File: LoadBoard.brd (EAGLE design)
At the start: 100 x 100 mm, 76 parts, among them IC1 7805TV, IC2 LM358D, IC3 MCP23S17SO, Q1 IRFZ44N, Q2 16MHz, T1 BC817, U1 ATMEGA328P_TQFP, U2 MAX232SOIC16

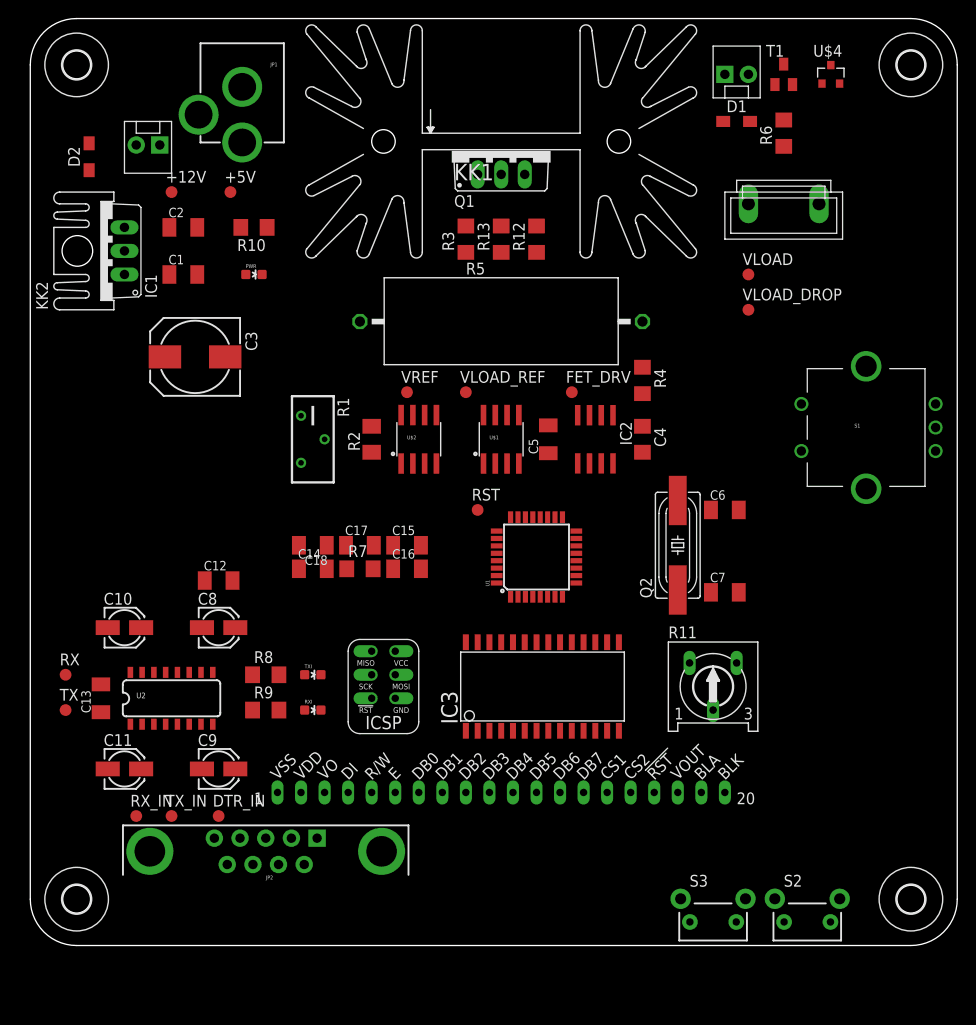
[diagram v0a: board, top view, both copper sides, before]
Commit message: routed first version of the board
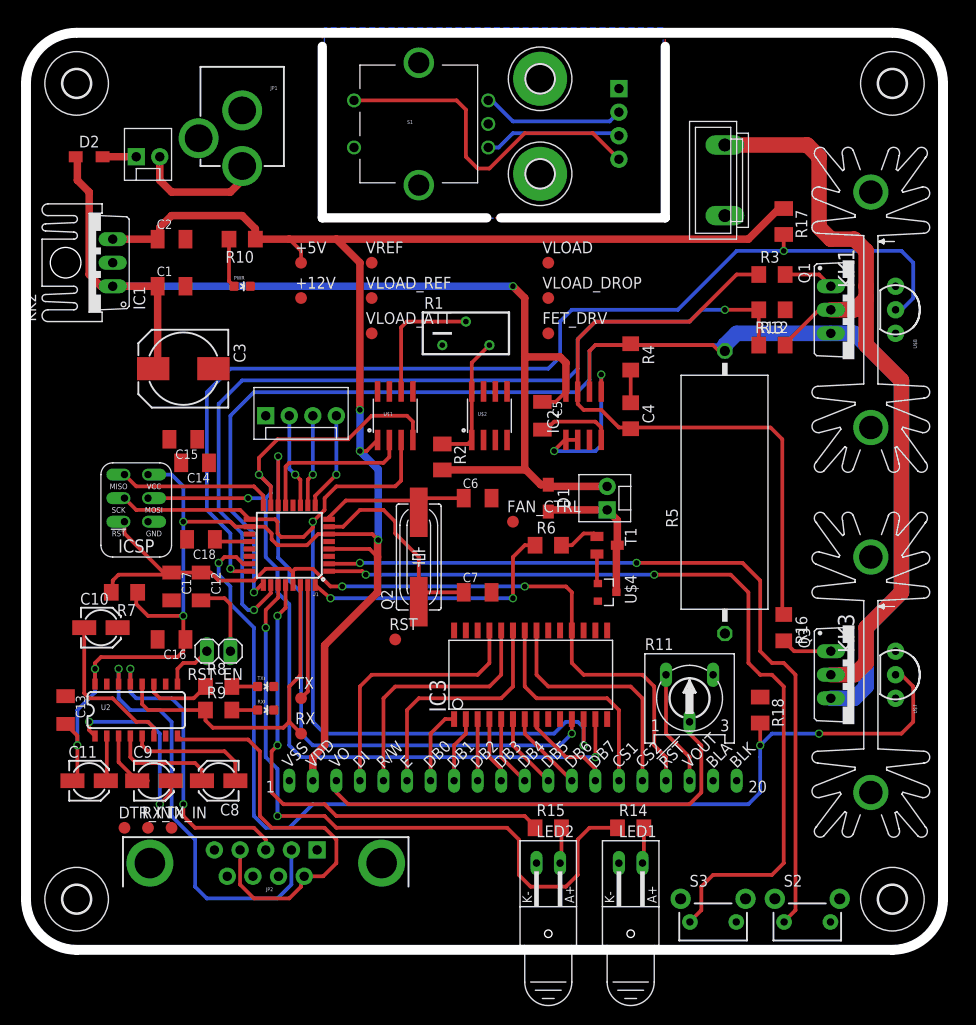
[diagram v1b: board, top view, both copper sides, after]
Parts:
- added ENCODER, JP3: (no value), SparkFun-Connectors:MOLEX-1X4
- added FAN_CTRL, VLOAD_ATT: TPB1,27, testpad:B1,27
- added H5, H6: 3MM, holes:3,0-PAD
- added KK3: SK104-PAD, heatsink:SK104-PAD
- added LED1, LED2: (no value), led:Q62902-B155
- added Q3: IRFZ44N, OwnStuff:TO-220-V
- added R14, R15, R16: 100, rcl:R1206
- added R17, R18: 4k7, rcl:M1206
- added RST_EN: (no value), pinhead:1X02
- added U$7, U$8: DS18B20, OwnStuff:TO-92
- KK1: value SK129 -> SK104-PAD; device heatsink:SK129-HOLE -> heatsink:SK104-PAD
- moved U$4 60.9 mm to (62.2, 38.1), turned to 270 degrees
- moved S1 58.3 mm to (41.9, 88.6)
- moved T1 54.3 mm to (62.2, 43.2), turned to 270 degrees
- moved R6 51.2 mm to (55.9, 43.2), turned to 0 degrees
- moved FAN 48.7 mm to (62.2, 47.0), turned to 90 degrees
- moved D1 45.4 mm to (55.9, 48.3), turned to 270 degrees
- moved KK1 44.9 mm to (91.4, 68.6), turned to 270 degrees
- moved Q1 38.4 mm to (86.4, 68.6), turned to 270 degrees
- moved R3 33.2 mm to (80.0, 72.4), turned to 0 degrees
- moved U$5 32.8 mm to (11.4, 48.3)
- moved R5 30.4 mm to (74.9, 48.9), turned to 90 degrees
- moved R13 30.2 mm to (80.0, 68.6), turned to 180 degrees
- moved Q2 28.0 mm to (41.9, 41.9)
- moved R12 27.9 mm to (80.0, 64.8), turned to 0 degrees
- moved C6 26.7 mm to (48.3, 48.3)
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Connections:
- new net GNDIO: JP3.1, S1.C, S1.SW-
- new net LED1: R14.1, U1.27
- new net LED2: R15.1, U1.28
- new net N$43: LED1.A, R14.2
- new net N$44: LED2.A, R15.2
- new net N$45: JP3.4, S1.SW+
- new net N$46: JP3.3, S1.A
- new net N$47: Q3.1, R16.2
- new net N$49: JP3.2, S1.B
- new net RST_EN: C12.2, RST_EN.1
- new net TH1: R18.2, U$7.2, U1.23
- new net TH2: R17.2, U$8.2, U1.24
- net +12V: now also FAN.2; no longer FAN.1
- net BTN_A: now also U1.2; no longer U1.1
- net BTN_B: now also U1.1; no longer U1.2
- net ENC_A: now also ENCODER.3; no longer S1.A
- net ENC_B: now also ENCODER.2; no longer S1.B
- net ENC_BTN: now also ENCODER.4; no longer S1.SW+
- net FAN: now also FAN_CTRL.TP
- net GND: now also ENCODER.1, LED1.K, LED2.K, U$7.1, U$8.1; no longer S1.C, S1.SW-
- net LOAD+: now also Q3.2
- net N$10: now also R16.1
- net N$12: now also DTR_IN.TP; no longer RX_IN.TP
- net N$13: now also RX_IN.TP; no longer DTR_IN.TP
- net N$26: now also PWR_SWITCH.2; no longer PWR_SWITCH.1
- net N$35: now also U$6.CS2; no longer U$6.DI
- net N$36: now also U$6.CS1; no longer U$6.RW
- net N$38: now also U$6.RW; no longer U$6.CS1
- net N$39: now also U$6.DI; no longer U$6.CS2
- net N$41: now also PWR_SWITCH.1; no longer PWR_SWITCH.2
- net N$5: now also FAN.1; no longer FAN.2
- net N$7: now also RST_EN.2; no longer C12.2
- net VCC: now also R17.1, R18.1, U$7.3, U$8.3
- net VLOAD_ATT: now also VLOAD_ATT.TP
- net VLOAD_DROP: now also Q3.3, U1.25
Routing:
- net VCC: track 0.00 -> 233.1 mm, vias 0 -> 7
- net VLOAD_DROP: track 0.00 -> 161.5 mm, vias 0 -> 1
- net +12V: track 0.00 -> 123.2 mm, vias 0 -> 2
- net TH1: track 0.00 -> 120.8 mm, vias 0 -> 3
- net TH2: track 0.00 -> 115.6 mm, vias 0 -> 2
- net MOSI: track 0.00 -> 107.8 mm, vias 0 -> 3
- net SCK: track 0.00 -> 97.2 mm, vias 0 -> 2
- net VLOAD_ATT: track 0.00 -> 95.8 mm, vias 0 -> 2
- net RST: track 0.00 -> 92.4 mm, vias 0 -> 2
- net BTN_B: track 0.00 -> 92.0 mm, vias 0 -> 2
- net LOAD+: track 0.00 -> 87.3 mm
- net BTN_A: track 0.00 -> 87.0 mm, vias 0 -> 2
- net LED1: track 0.00 -> 72.9 mm, vias 0 -> 2
- net N$10: track 0.00 -> 72.1 mm
- net CS1: track 0.00 -> 68.1 mm, vias 0 -> 2
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- added copper zone on layer 1, net GNDIO
- added copper zone on layer 16, net GNDIO
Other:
- board size 100 x 100 mm -> 99 x 99 mm
